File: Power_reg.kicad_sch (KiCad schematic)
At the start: 20 parts, among them J6 Conn_01x02_Female, U5 LMR36510ADDA

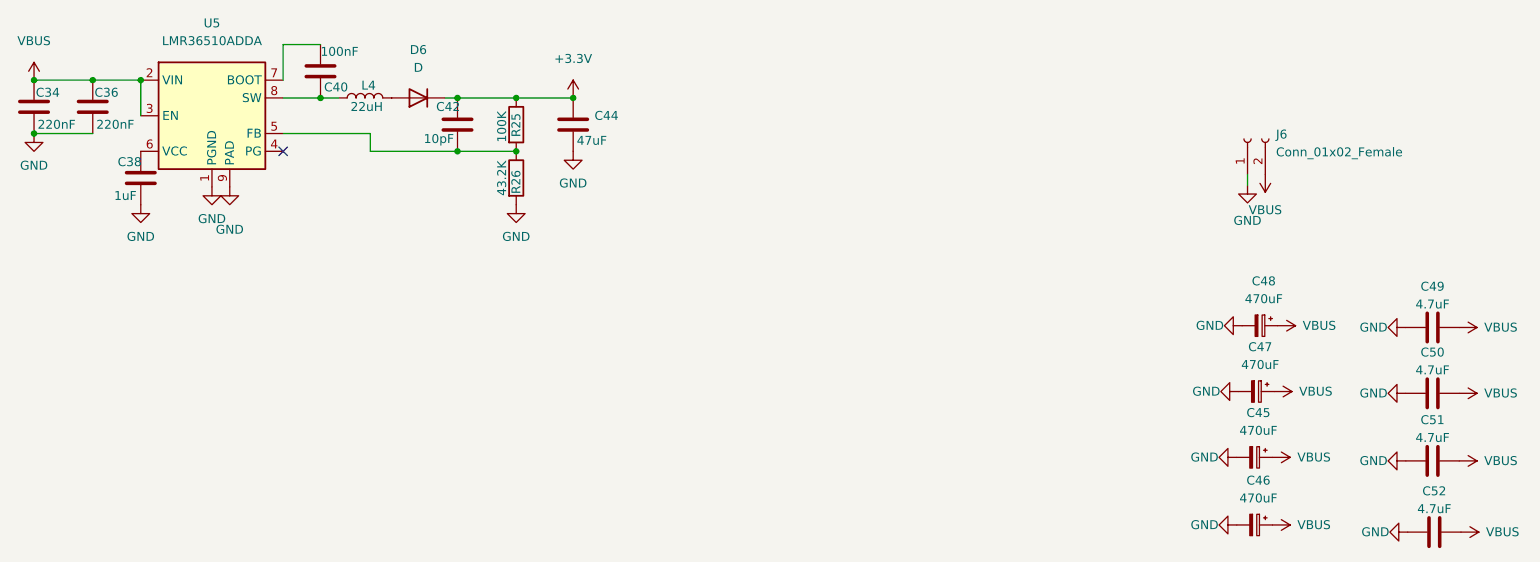
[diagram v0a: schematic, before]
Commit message: init routing done
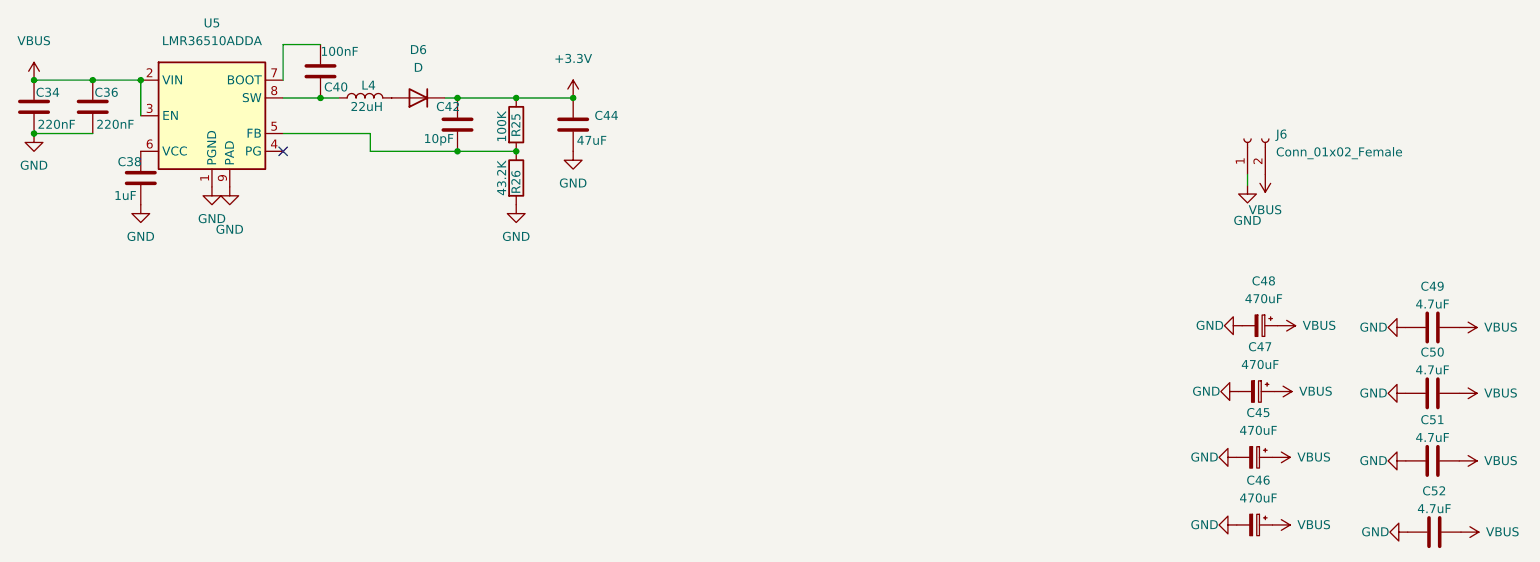
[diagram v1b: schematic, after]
